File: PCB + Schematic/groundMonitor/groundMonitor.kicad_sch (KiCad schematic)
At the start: 16 parts, among them J1 FTDI, J2 FTDI, SW1 Boot, SW2 Boot, SW3 Reset, SW4 Reset, U1 ESP32-MINI-1-N4, U2 ESP32-C3-WROOM-02-N4, U3 ESP32-C3-MINI-1-N4

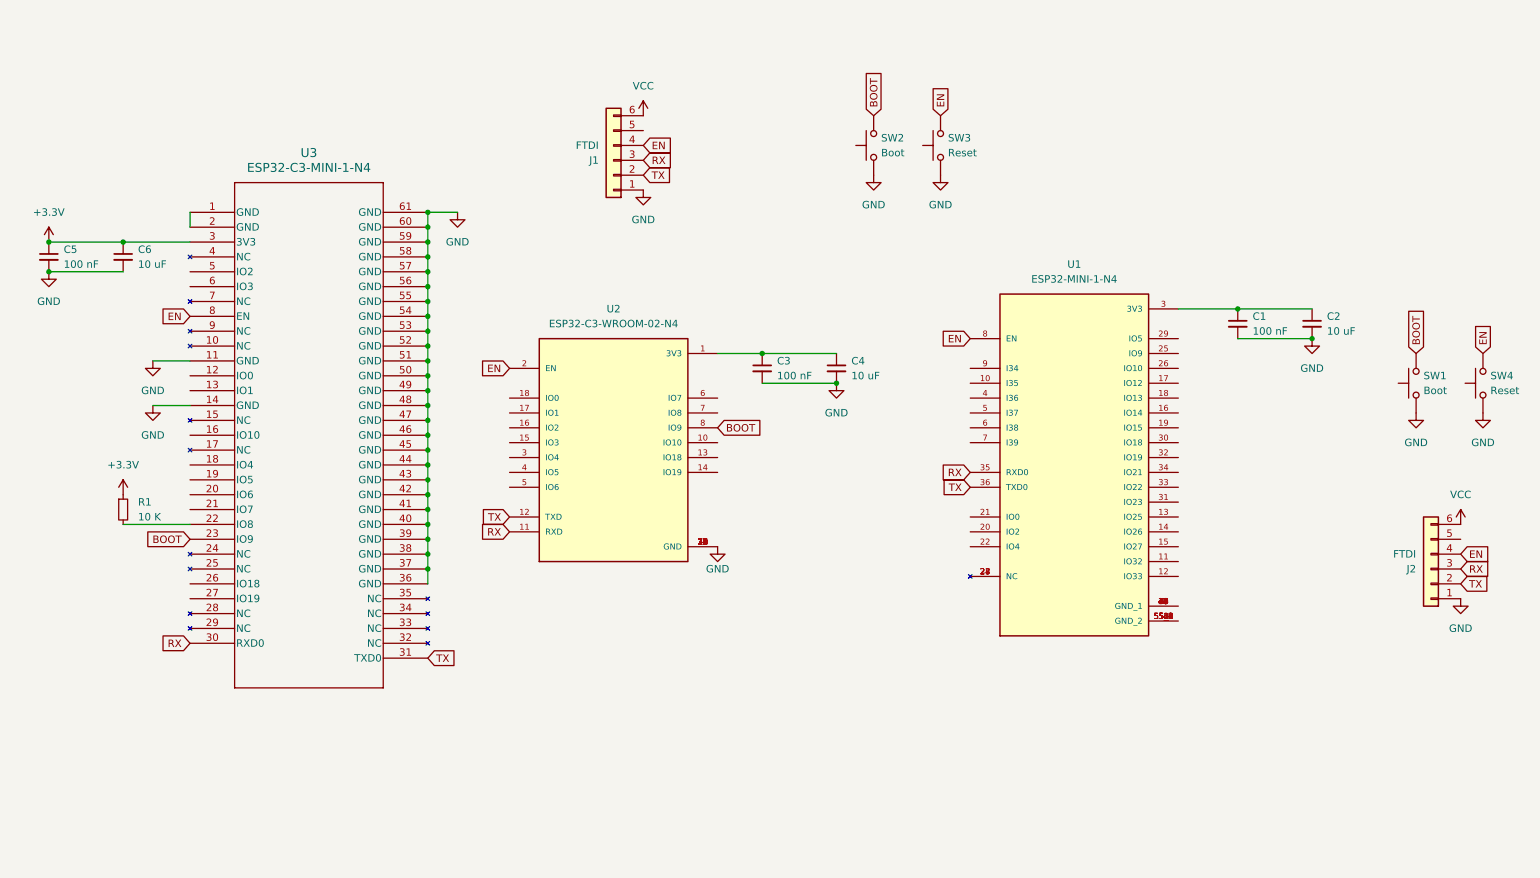
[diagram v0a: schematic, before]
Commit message: PCB
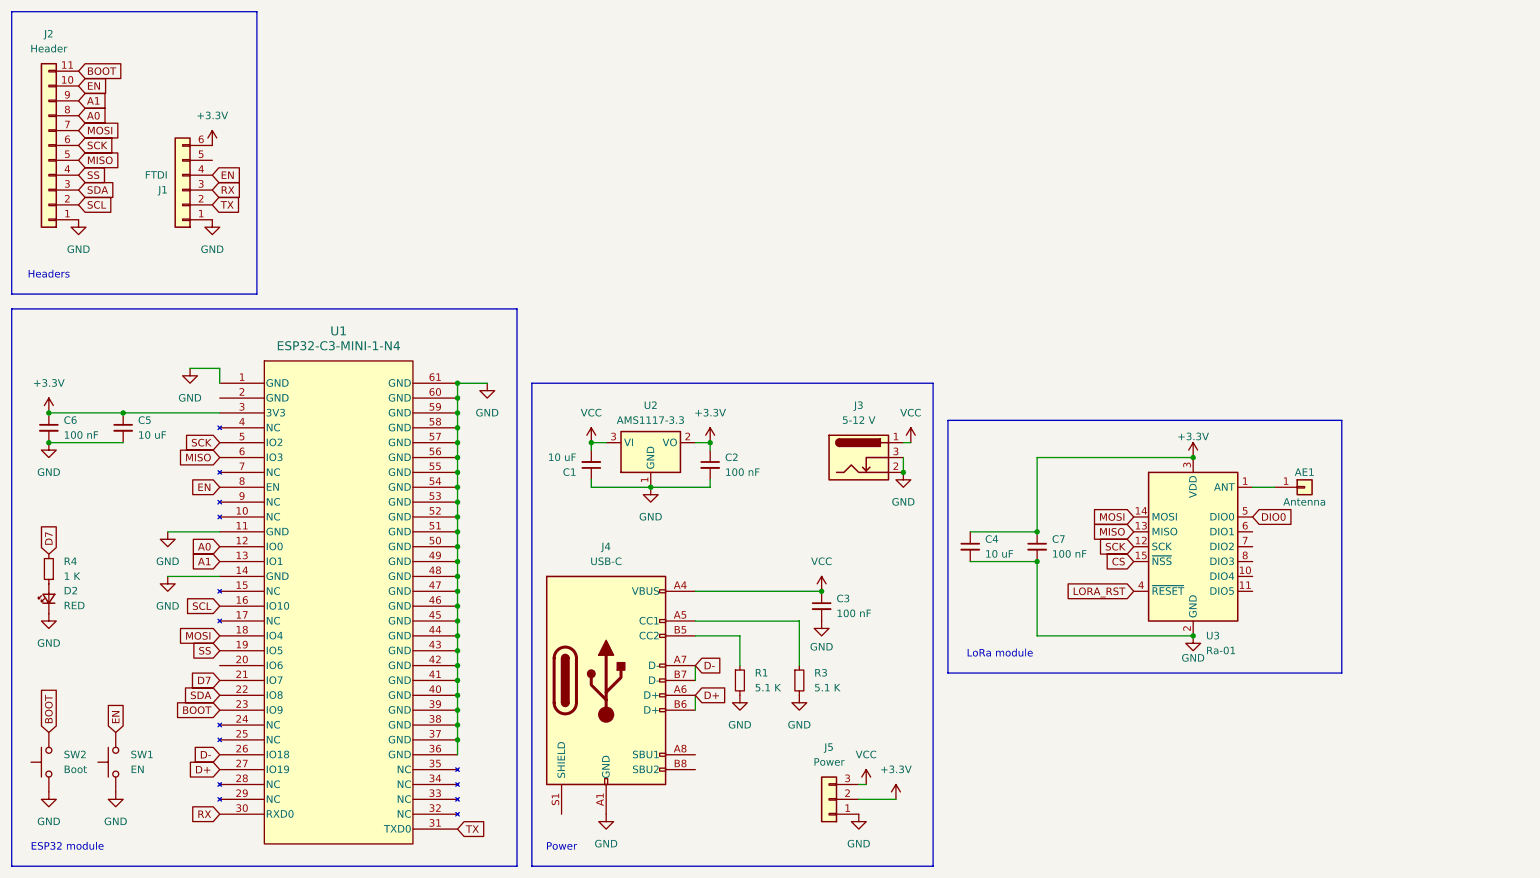
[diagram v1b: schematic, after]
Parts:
- removed J2: FTDI, symbol Connector_Generic:Conn_01x06
- removed SW3, SW4: Reset, symbol Switch:SW_Push
- removed U1: ESP32-MINI-1-N4, ESP32-MINI-1-N4:XCVR_ESP32-MINI-1-N4, symbol ESP32-MINI-1-N4:ESP32-MINI-1-N4
- removed U2: ESP32-C3-WROOM-02-N4, ESP32-C3-WROOM-02-N4:MODULE_ESP32-C3-WROOM-02-H4, symbol ESP32-C3-WROOM-02-N4:ESP32-C3-WROOM-02-N4
- removed U3: ESP32-C3-MINI-1-N4, ESP32-C3-MINI-1_EXP, symbol ESP32-MINI-1-N4-New:ESP32-C3-MINI-1-N4
- added AE1: Antenna, Connector_PinHeader_2.54mm:PinHeader_1x01_P2.54mm_Vertical, symbol Connector_Generic:Conn_01x01
- added C7: 100 nF, Capacitor_SMD:C_0603_1608Metric, symbol Device:C_Small
- added D2: RED, LED_SMD:LED_0603_1608Metric, symbol Device:LED_Small
- added J2: Header, Connector_PinHeader_2.54mm:PinHeader_1x11_P2.54mm_Vertical, symbol Connector_Generic:Conn_01x11
- added J3: 5-12 V, Connector_BarrelJack:BarrelJack_Horizontal, symbol Connector:Barrel_Jack_Switch
- added J4: USB-C, Connector_USB:USB_C_Receptacle_GCT_USB4105-xx-A_16P_TopMnt_Horizontal, symbol Connector:USB_C_Receptacle_USB2.0
- added J5: Power, Connector_PinHeader_2.54mm:PinHeader_1x03_P2.54mm_Vertical, symbol Connector_Generic:Conn_01x03
- added R3: 5.1 K, Resistor_SMD:R_0402_1005Metric, symbol Device:R_Small
- added R4: 1 K, Resistor_SMD:R_0402_1005Metric, symbol Device:R_Small
- added U1: ESP32-C3-MINI-1-N4, ESP32-C3-MINI-1-N4:ESP32-C3-MINI-1_EXP, symbol ESP32-MINI-1-N4-New:ESP32-C3-MINI-1-N4
- added U2: AMS1117-3.3, Package_TO_SOT_SMD:SOT-223-3_TabPin2, symbol Regulator_Linear:AMS1117-3.3
- added U3: Ra-01, RF_Module:Ai-Thinker-Ra-01-LoRa, symbol RF_Module:Ai-Thinker-Ra-01
- C1, C5: value 100 nF -> 10 uF; footprint (none) -> Capacitor_SMD:C_0603_1608Metric; LCSC (none) -> C19702
- C2, C6: value 10 uF -> 100 nF; footprint (none) -> Capacitor_SMD:C_0603_1608Metric; LCSC (none) -> C14663
- C3: footprint (none) -> Capacitor_SMD:C_0603_1608Metric; LCSC (none) -> C14663
- C4: footprint (none) -> Capacitor_SMD:C_0603_1608Metric; LCSC (none) -> C19702
- J1: footprint (none) -> Connector_PinHeader_2.54mm:PinHeader_1x06_P2.54mm_Vertical
- R1: value 10 K -> 5.1 K; footprint (none) -> Resistor_SMD:R_0402_1005Metric; LCSC (none) -> C25905
- SW1: value Boot -> EN; footprint (none) -> Button_Switch_SMD:SW_SPST_CK_RS282G05A3; LCSC (none) -> C2888954
- SW2: footprint (none) -> Button_Switch_SMD:SW_SPST_CK_RS282G05A3; LCSC (none) -> C2888954
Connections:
- net +3.3V: now also C2.1, C4.1, J1.6 (Pin_6), C7.1, J5.2 (Pin_2), U1.3 (3V3), U2.2 (VO), U3.3 (VDD); no longer R1.1
- net BOOT: now also J2.11 (Pin_11), U1.23 (IO9); no longer SW1.2
- net EN: now also SW1.2, J2.10 (Pin_10), U1.8 (EN)
- net GND: now also C1.1, R1.2, C7.2, D2.1 (K), J2.1 (Pin_1), J3.2, J3.3, J4.A1 (GND), J4.A12 (GND), J4.B1 (GND), J4.B12 (GND), J5.1 (Pin_1), R3.2, U1.1 (GND), U1.11 (GND), U1.14 (GND), U1.36 (GND), U1.37 (GND), U1.38 (GND), U1.39 (GND), U1.40 (GND), U1.41 (GND), U1.42 (GND), U1.43 (GND), U1.44 (GND), U1.45 (GND), U1.46 (GND), U1.47 (GND), U1.48 (GND), U1.49 (GND), U1.50 (GND), U1.51 (GND), U1.52 (GND), U1.53 (GND), U1.54 (GND), U1.55 (GND), U1.56 (GND), U1.57 (GND), U1.58 (GND), U1.59 (GND), U1.60 (GND), U1.61 (GND), U2.1 (GND), U3.16 (GND), U3.2 (GND), U3.9 (GND); no longer C1.2
- net RX: now also U1.30 (RXD0)
- net TX: now also U1.31 (TXD0)
- net VCC: now also C1.2, C3.1, J3.1, J4.A4 (VBUS), J4.A9 (VBUS), J4.B4 (VBUS), J4.B9 (VBUS), J5.3 (Pin_3), U2.3 (VI); no longer J1.6 (Pin_6)
- new net: D2.2 (A), R4.1
- new net: J4.B5 (CC2), R1.1
- new net: J4.A5 (CC1), R3.1
- new net: AE1.1 (Pin_1), U3.1 (ANT)
- new net A0: J2.8 (Pin_8), U1.12 (IO0)
- new net A1: J2.9 (Pin_9), U1.13 (IO1)
- new net CS: U3.15 (~{NSS})
- new net D+: J4.A6 (D+), J4.B6 (D+), U1.27 (IO19)
- new net D-: J4.A7 (D-), J4.B7 (D-), U1.26 (IO18)
- new net D7: R4.2, U1.21 (IO7)
- new net DIO0: U3.5 (DIO0)
- new net LORA_RST: U3.4 (~{RESET})
- new net MISO: J2.5 (Pin_5), U1.6 (IO3), U3.13 (MISO)
- new net MOSI: J2.7 (Pin_7), U1.18 (IO4), U3.14 (MOSI)
- new net SCK: J2.6 (Pin_6), U1.5 (IO2), U3.12 (SCK)
- new net SCL: J2.2 (Pin_2), U1.16 (IO10)
- new net SDA: J2.3 (Pin_3), U1.22 (IO8)
- new net SS: J2.4 (Pin_4), U1.19 (IO5)
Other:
- note added: "ESP32 module"
- note added: "Headers"
- note added: "LoRa module"
- note added: "Power"
- moved on the sheet: J1

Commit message: More PCB
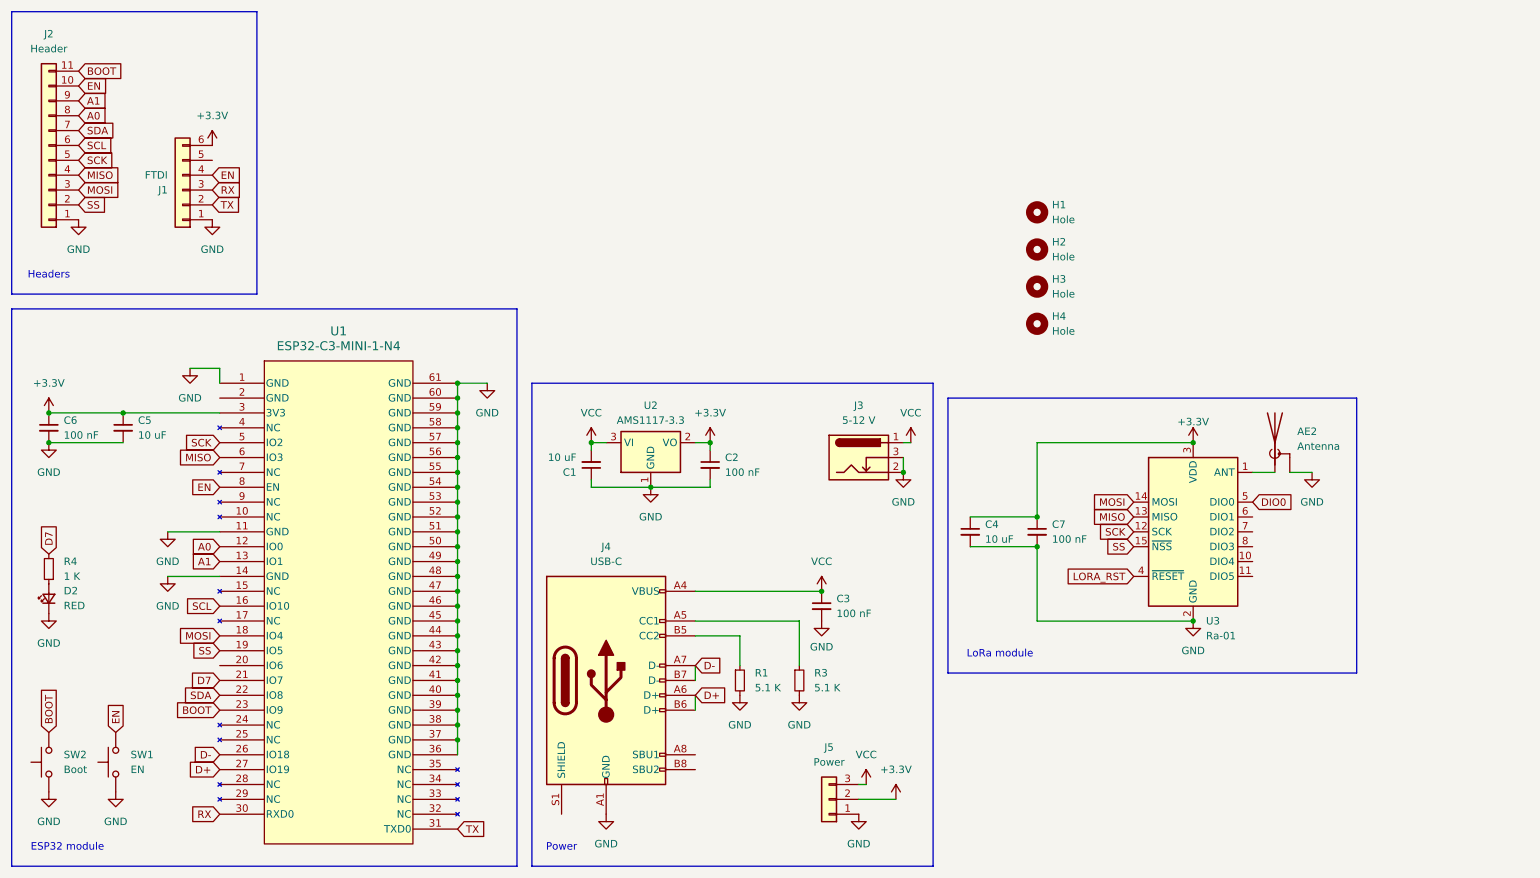
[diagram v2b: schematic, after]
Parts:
- removed AE1: Antenna, Connector_PinHeader_2.54mm:PinHeader_1x01_P2.54mm_Vertical, symbol Connector_Generic:Conn_01x01
- added AE2: Antenna, Connector_Coaxial:SMA_Amphenol_132289_EdgeMount, symbol Device:Antenna_Shield
- added H1, H2, H3, H4: Hole, MountingHole:MountingHole_3.2mm_M3, symbol Mechanical:MountingHole
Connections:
- net CS is gone; now on net SS: U3.15 (~{NSS})
- net GND: now also AE2.2 (Shield)
- net MISO: now also J2.4 (Pin_4); no longer J2.5 (Pin_5)
- net MOSI: now also J2.3 (Pin_3); no longer J2.7 (Pin_7)
- net SCK: now also J2.5 (Pin_5); no longer J2.6 (Pin_6)
- net SCL: now also J2.6 (Pin_6); no longer J2.2 (Pin_2)
- net SDA: now also J2.7 (Pin_7); no longer J2.3 (Pin_3)
- net SS: now also J2.2 (Pin_2); no longer J2.4 (Pin_4)
- net at U3.1 (ANT): now also AE2.1 (A)
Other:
- moved on the sheet: C4, C7, U3
